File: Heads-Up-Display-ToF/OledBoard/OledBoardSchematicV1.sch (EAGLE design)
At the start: 46 parts, among them U1 AP3012, U2 UG-2856KLBAG01_4WSPI, U3 ATMEGA328P_TQFP, U4 CH340C

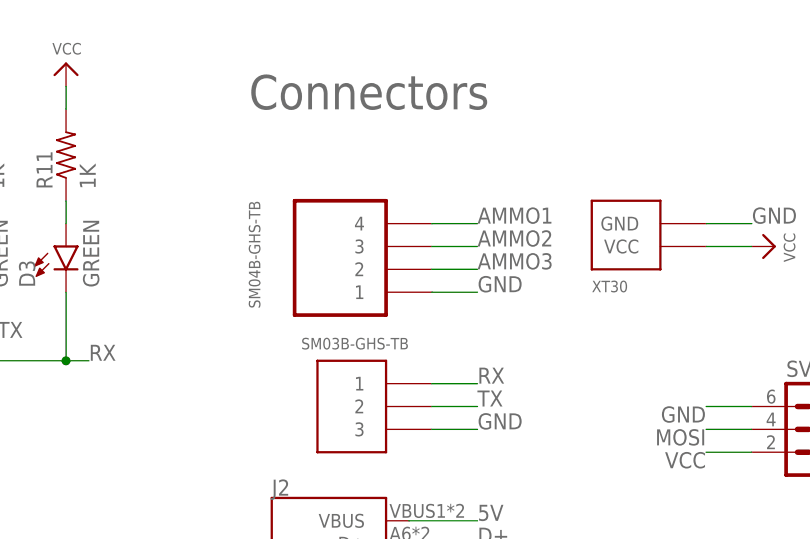
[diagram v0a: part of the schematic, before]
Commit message: added changes that were left behind
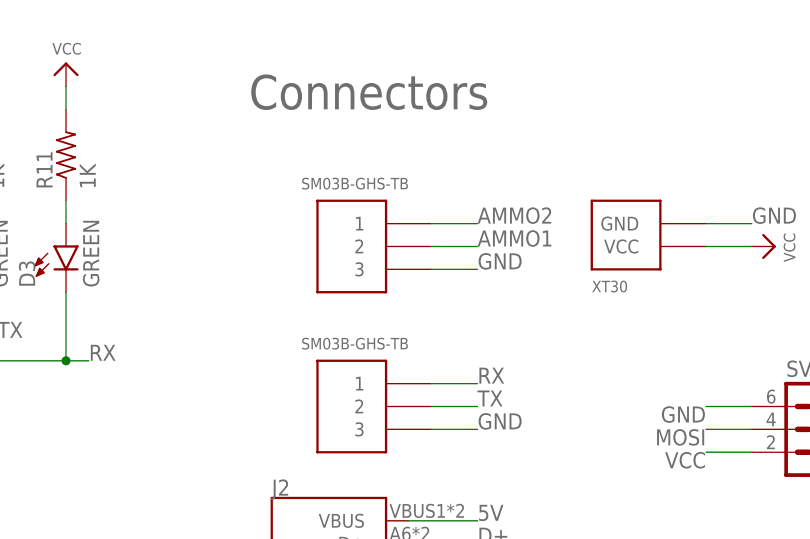
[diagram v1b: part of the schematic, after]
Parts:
- U$5: value SM04B-GHS-TB -> SM03B-GHS-TB; device oledBoard:SM04B-GHS-TB -> oledBoard:SM03B-GHS-TB
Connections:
- net AMMO1: now also U$5.2; no longer U$5.4
- net AMMO2: now also U$5.1; no longer U$5.3
- net AMMO3: no longer U$5.2
- net GND: now also U$5.3; no longer U$5.1
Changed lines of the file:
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@@
 <part name="C6" library="SparkFun-Capacitors" library_urn="urn:adsk.eagle:library:510" deviceset="0.1UF" device="-0603-25V-(+80/-20%)" package3d_urn="urn:adsk.eagle:package:37414/1" value="0.1uF"/>
 <part name="C1" library="SparkFun-Capacitors" library_urn="urn:adsk.eagle:library:510" deviceset="0.1UF" device="-0603-25V-(+80/-20%)" package3d_urn="urn:adsk.eagle:package:37414/1" value="0.1uF"/>
-<part name="U$5" library="oledBoard" deviceset="SM04B-GHS-TB" device=""/>
 <part name="R5" library="rcl" library_urn="urn:adsk.eagle:library:334" deviceset="R-US_" device="R0603" package3d_urn="urn:adsk.eagle:package:23555/3" value="1K"/>
 <part name="R6" library="rcl" library_urn="urn:adsk.eagle:library:334" deviceset="R-US_" device="R0603" package3d_urn="urn:adsk.eagle:package:23555/3" value="1k"/>
@@
 <part name="U$7" library="HenrySilva" deviceset="MDKK1616T2R2MM" device="" value="2.2uH/NRH2412T2R2MNGH"/>
 <part name="SV1" library="con-lstb" library_urn="urn:adsk.eagle:library:162" deviceset="MA03-2" device="" package3d_urn="urn:adsk.eagle:package:8334/1"/>
+<part name="U$5" library="oledBoard" deviceset="SM03B-GHS-TB" device=""/>
 </parts>
 <sheets>
@@
 <attribute name="VALUE" x="62.484" y="2.921" size="1.778" layer="96" font="vector"/>
 </instance>
-<instance part="U$5" gate="G$1" x="96.52" y="121.92" smashed="yes" rot="R270"/>
 <instance part="R5" gate="G$1" x="35.56" y="35.56" smashed="yes" rot="R90">
 <attribute name="NAME" x="34.0614" y="31.75" size="1.778" layer="95" rot="R90"/>
@@
 <attribute name="NAME" x="151.13" y="102.362" size="1.778" layer="95"/>
 </instance>
+<instance part="U$5" gate="G$1" x="106.68" y="121.92" smashed="yes" rot="R180"/>
 </instances>
 <busses>
@@
 </segment>
 <segment>
-<pinref part="U$5" gate="G$1" pin="1"/>
-<wire x1="111.76" y1="111.76" x2="116.84" y2="111.76" width="0.1524" layer="91"/>
-<label x="116.84" y="111.76" size="1.778" layer="95"/>
-</segment>
-<segment>
 <pinref part="U5" gate="G$1" pin="GND"/>
 <wire x1="223.52" y1="10.16" x2="218.44" y2="10.16" width="0.1524" layer="91"/>
@@
 <wire x1="147.32" y1="99.06" x2="142.24" y2="99.06" width="0.1524" layer="91"/>
 <label x="142.24" y="99.06" size="1.778" layer="95" rot="R180"/>
+</segment>
+<segment>
+<pinref part="U$5" gate="G$1" pin="3"/>
+<wire x1="111.76" y1="114.3" x2="116.84" y2="114.3" width="0.1524" layer="91"/>
+<label x="116.84" y="114.3" size="1.778" layer="95"/>
 </segment>
 </net>
@@
 <net name="AMMO1" class="0">
 <segment>
-<wire x1="111.76" y1="119.38" x2="116.84" y2="119.38" width="0.1524" layer="91"/>
-<label x="116.84" y="119.38" size="1.778" layer="95"/>
-<pinref part="U$5" gate="G$1" pin="4"/>
-</segment>
-<segment>
 <pinref part="U3" gate="U1" pin="PC2(ADC2)"/>
 <wire x1="15.24" y1="33.02" x2="20.32" y2="33.02" width="0.1524" layer="91"/>
 <label x="20.32" y="33.02" size="1.778" layer="95"/>
 </segment>
+<segment>
+<pinref part="U$5" gate="G$1" pin="2"/>
+<wire x1="111.76" y1="116.84" x2="116.84" y2="116.84" width="0.1524" layer="91"/>
+<label x="116.84" y="116.84" size="1.778" layer="95"/>
+</segment>
 </net>
 <net name="AMMO2" class="0">
@@
 </segment>
 <segment>
-<wire x1="111.76" y1="116.84" x2="116.84" y2="116.84" width="0.1524" layer="91"/>
-<label x="116.84" y="116.84" size="1.778" layer="95"/>
-<pinref part="U$5" gate="G$1" pin="3"/>
+<pinref part="U$5" gate="G$1" pin="1"/>
+<wire x1="111.76" y1="119.38" x2="116.84" y2="119.38" width="0.1524" layer="91"/>
+<label x="116.84" y="119.38" size="1.778" layer="95"/>
 </segment>
 </net>
 <net name="AMMO3" class="0">
 <segment>
-<pinref part="U$5" gate="G$1" pin="2"/>
-<wire x1="111.76" y1="114.3" x2="116.84" y2="114.3" width="0.1524" layer="91"/>
-<label x="116.84" y="114.3" size="1.778" layer="95"/>
-</segment>
-<segment>
 <pinref part="U3" gate="U1" pin="PC0(ADC0)"/>
